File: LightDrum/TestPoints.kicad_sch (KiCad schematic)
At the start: 6 parts

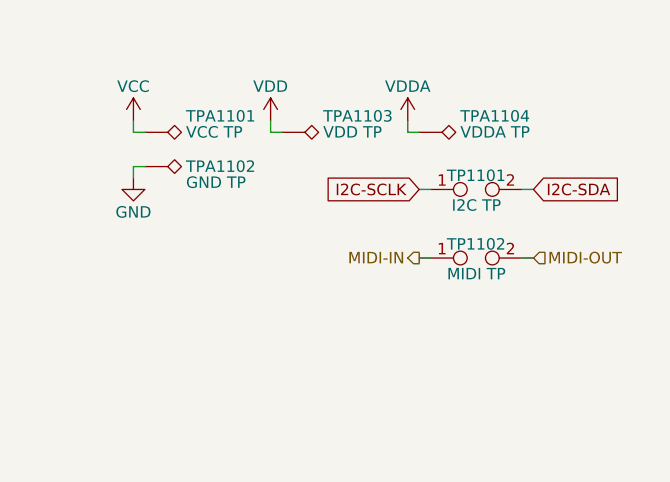
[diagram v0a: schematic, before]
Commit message: interface layout completed - REV6
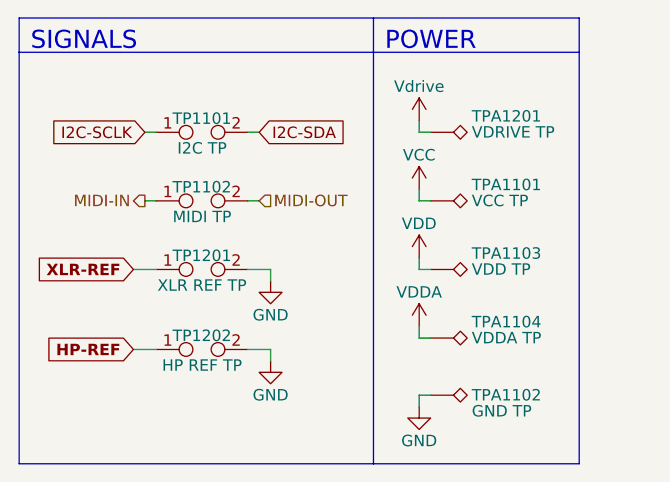
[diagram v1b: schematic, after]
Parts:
- added TP1201: XLR REF TP, Connector_PinHeader_2.54mm:PinHeader_1x02_P2.54mm_Vertical, symbol Connector:TestPoint_2Pole
- added TP1202: HP REF TP, Connector_PinHeader_2.54mm:PinHeader_1x02_P2.54mm_Vertical, symbol Connector:TestPoint_2Pole
- added TPA1201: VDRIVE TP, TestPoint:TestPoint_Loop_D2.54mm_Drill1.5mm_Beaded, symbol Connector:TestPoint_Alt
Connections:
- net GND: now also TP1201.2, TP1202.2
- new net HP-REF: TP1202.1
- new net Vdrive: TPA1201.1
- new net XLR-REF: TP1201.1
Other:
- note added: "POWER"
- note added: "SIGNALS"
- moved on the sheet: TP1101, TP1102, TPA1101, TPA1102, TPA1103, TPA1104
